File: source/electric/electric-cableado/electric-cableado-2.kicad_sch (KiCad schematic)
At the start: 111 parts

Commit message: 22/01/2025 Update
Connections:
- net at V1.: now also S2.; no longer S1.
- net at S2.: now also L1.; no longer V1.
- net at L2.: now also S2.; no longer S1.
- net at S1., S2.: no longer L1.
- net at S1.: now also L1., S2.; no longer V1.
- net at S1.: now also L2., S2.; no longer V1.
- net at L2., S2.: now also L1.; no longer S1.
- new net: L1., L2., V1. (x2)
- new net: S1., V1. (x3)
- new net: L2., S1.
- new net: L1., S1., S2.

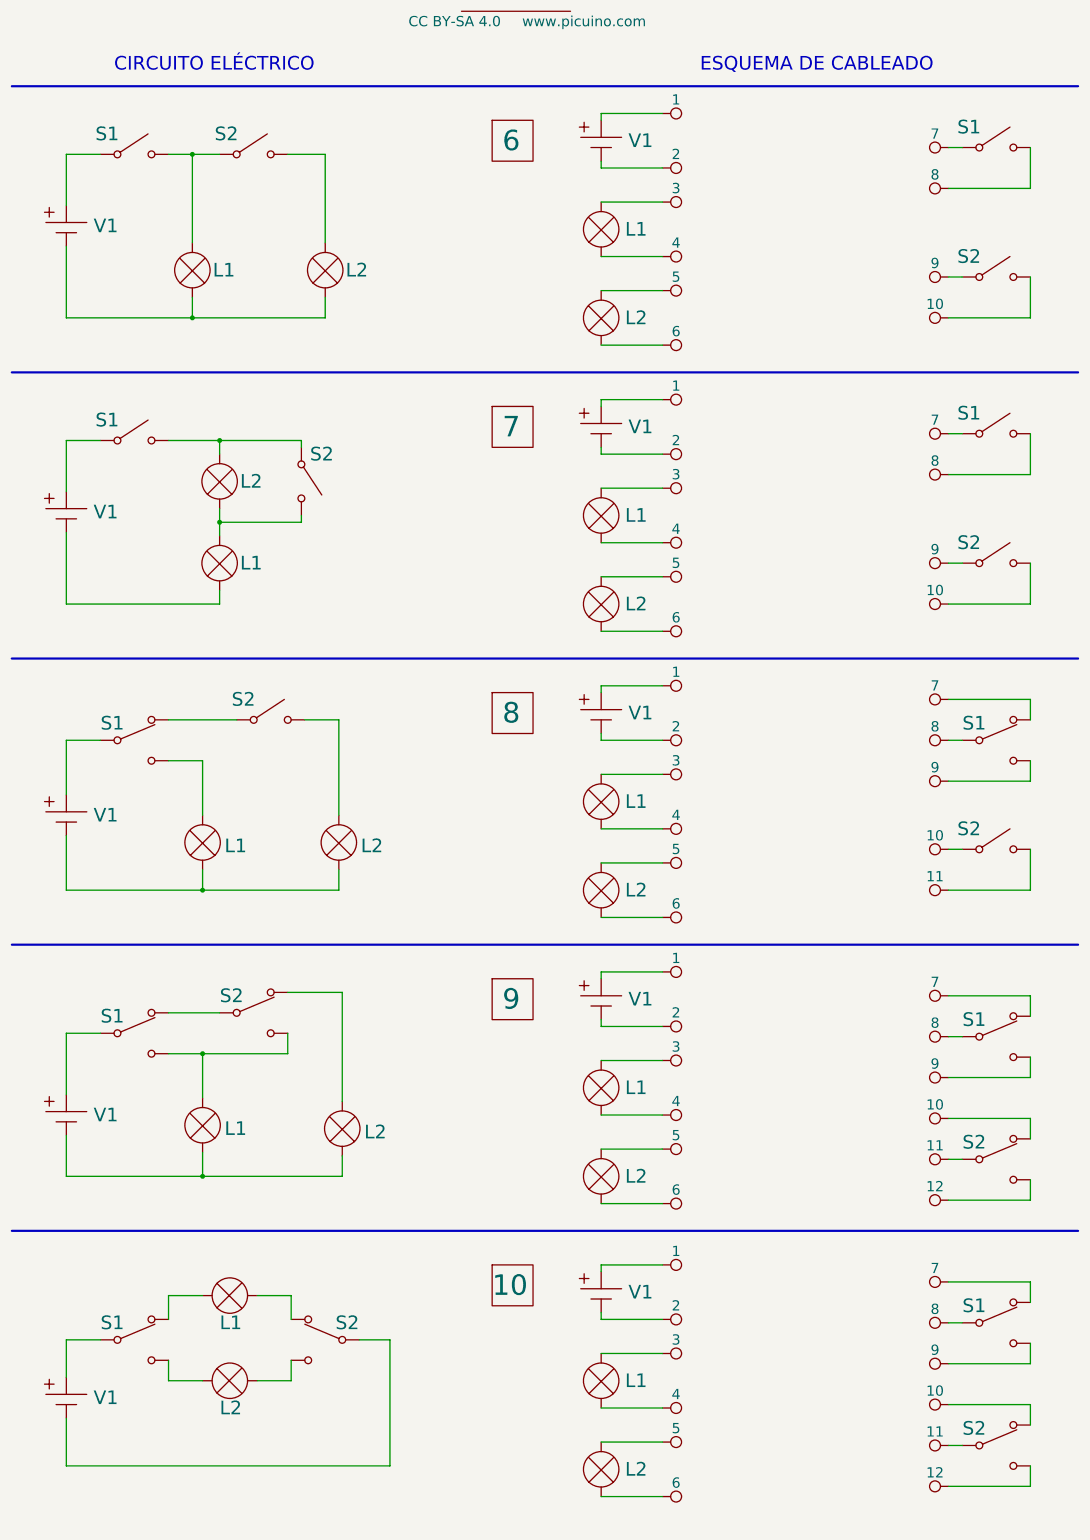
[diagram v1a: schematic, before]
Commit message: 25/01/2025 Update
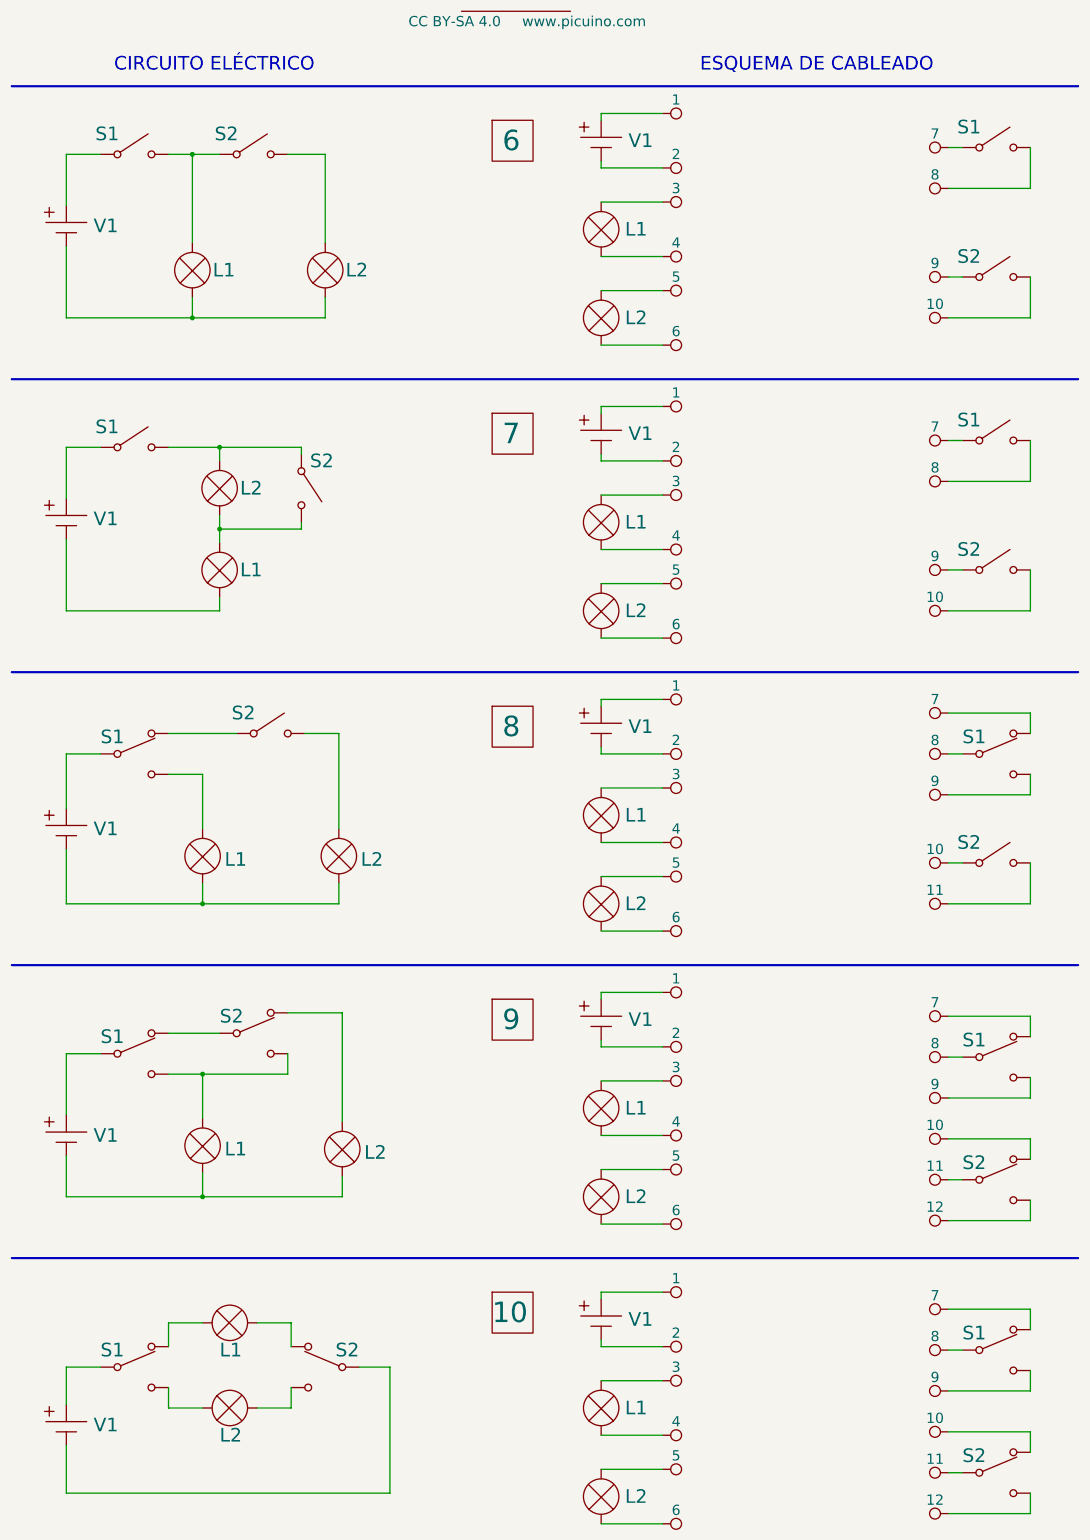
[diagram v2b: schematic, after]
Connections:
- net at V1.: now also S2.; no longer S1.
- net at S2.: now also L1.; no longer V1.
- net at L2.: now also S2.; no longer S1.
- net at S1., S2.: no longer L1.
- net at S1.: now also L1., S2.; no longer V1.
- net at S1.: now also L2., S2.; no longer V1.
- net at L2., S2.: now also L1.; no longer S1.
- new net: L1., L2., V1. (x2)
- new net: S1., V1. (x3)
- new net: L2., S1.
- new net: L1., S1., S2.
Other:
- moved on the sheet: L1, L2, S1, S2, V1
